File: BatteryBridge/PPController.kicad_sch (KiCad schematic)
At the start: 18 parts, among them Q401 BSS84LT1G, Q402 BSS84LT1G, U401 LTC4412xS6, U402 LTC4412xS6

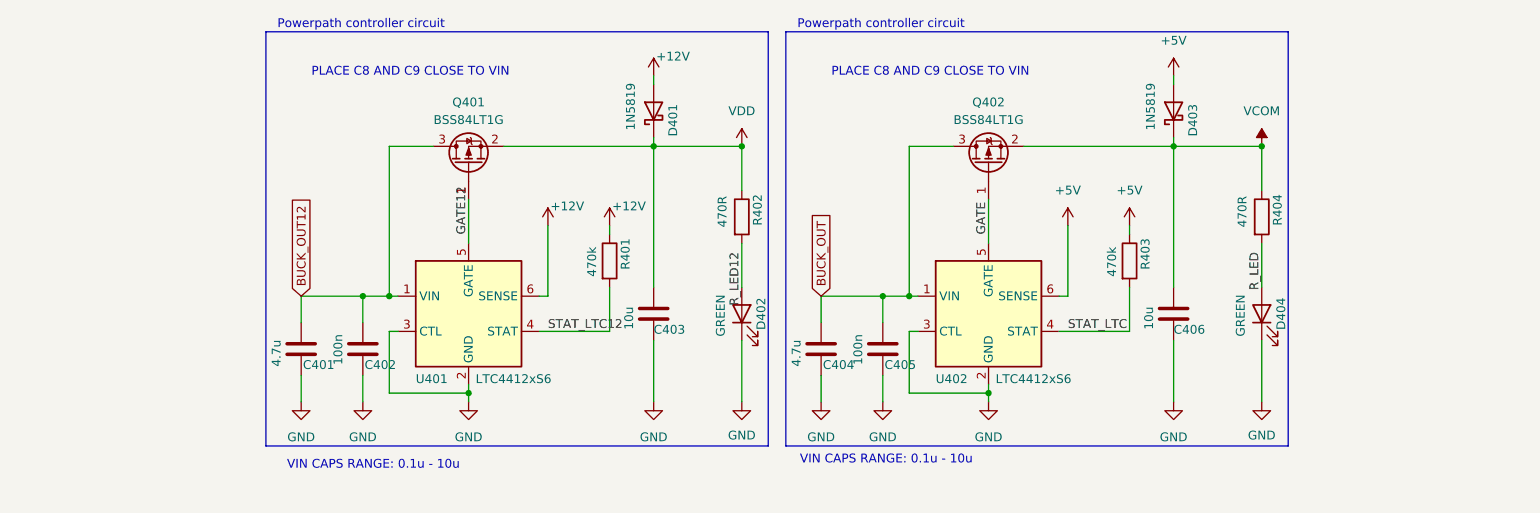
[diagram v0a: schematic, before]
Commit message: Finished v1.2, added gerbers
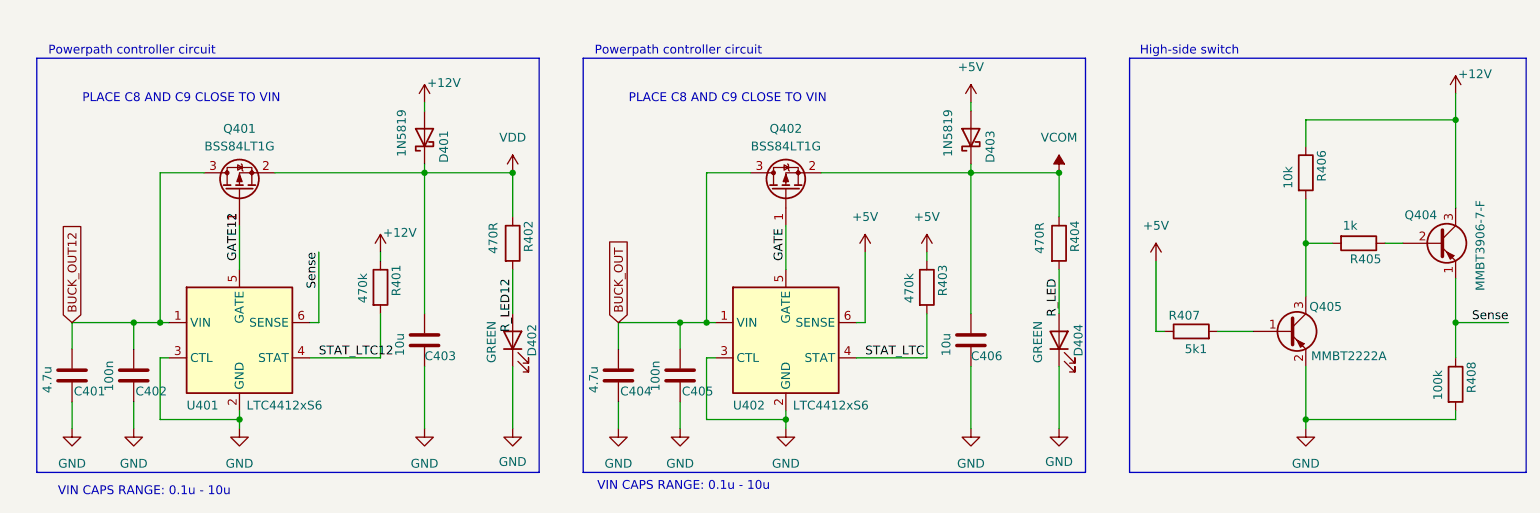
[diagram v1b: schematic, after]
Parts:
- added Q404: MMBT3906-7-F, Package_TO_SOT_SMD:SOT-23-3, symbol Device:Q_PNP_EBC
- added Q405: MMBT2222A, Package_TO_SOT_SMD:SOT-23-3, symbol Device:Q_PNP_BEC
- added R405: 1k, Resistor_SMD:R_0805_2012Metric, symbol Device:R
- added R406: 10k, Resistor_SMD:R_0805_2012Metric, symbol Device:R
- added R407: 5k1, Resistor_SMD:R_0805_2012Metric, symbol Device:R
- added R408: 100k, Resistor_SMD:R_0805_2012Metric, symbol Device:R
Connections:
- net +12V: now also Q404.3 (C), R406.1; no longer U401.6 (SENSE)
- net +5V: now also R407.1
- net GND: now also Q405.2 (E), R408.2
- new net: Q405.3 (C), R405.2, R406.2
- new net: Q404.2 (B), R405.1
- new net: Q405.1 (B), R407.2
- new net Sense: Q404.1 (E), R408.1, U401.6 (SENSE)
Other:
- note added: "High-side switch"
- moved on the sheet: C401, C402, C403, C404, C405, C406, D401, D402, D403, D404, Q401, Q402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
